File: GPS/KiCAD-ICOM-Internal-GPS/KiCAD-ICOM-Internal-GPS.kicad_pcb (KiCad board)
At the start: 2 copper layers, 20 x 35 mm, 2 parts, among them J1 ICOM-J1, U1 MAX-M10M-00B

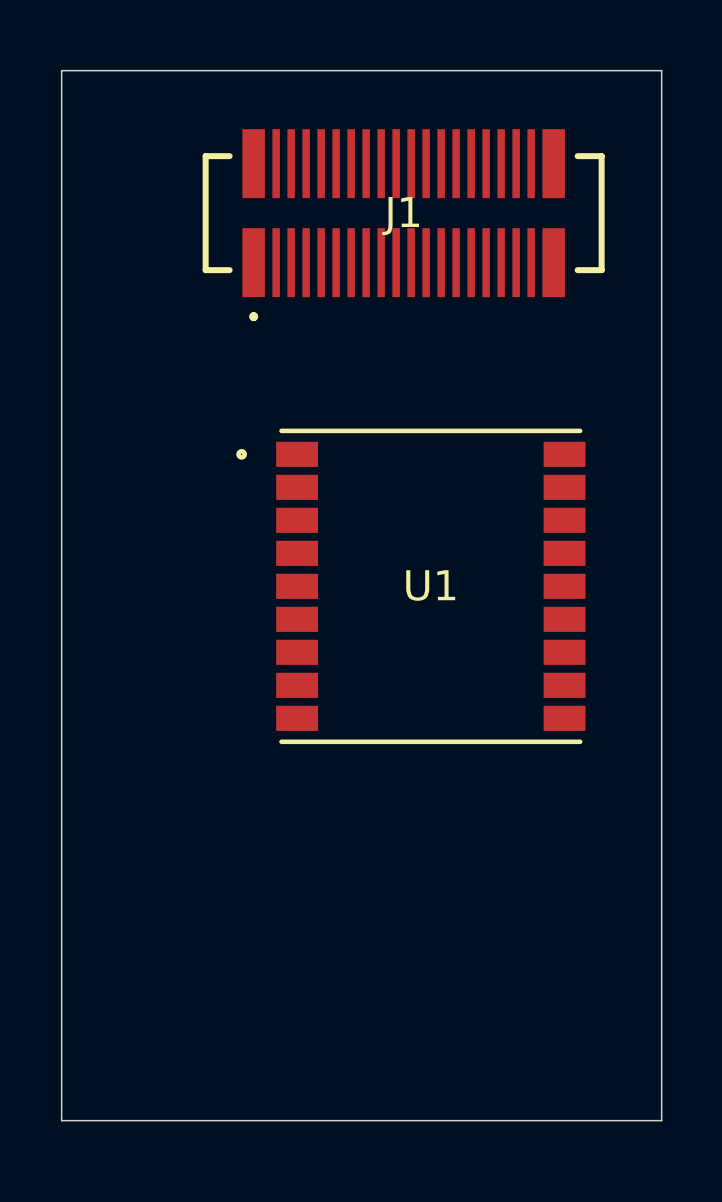
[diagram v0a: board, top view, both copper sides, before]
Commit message: updated v1.0 design
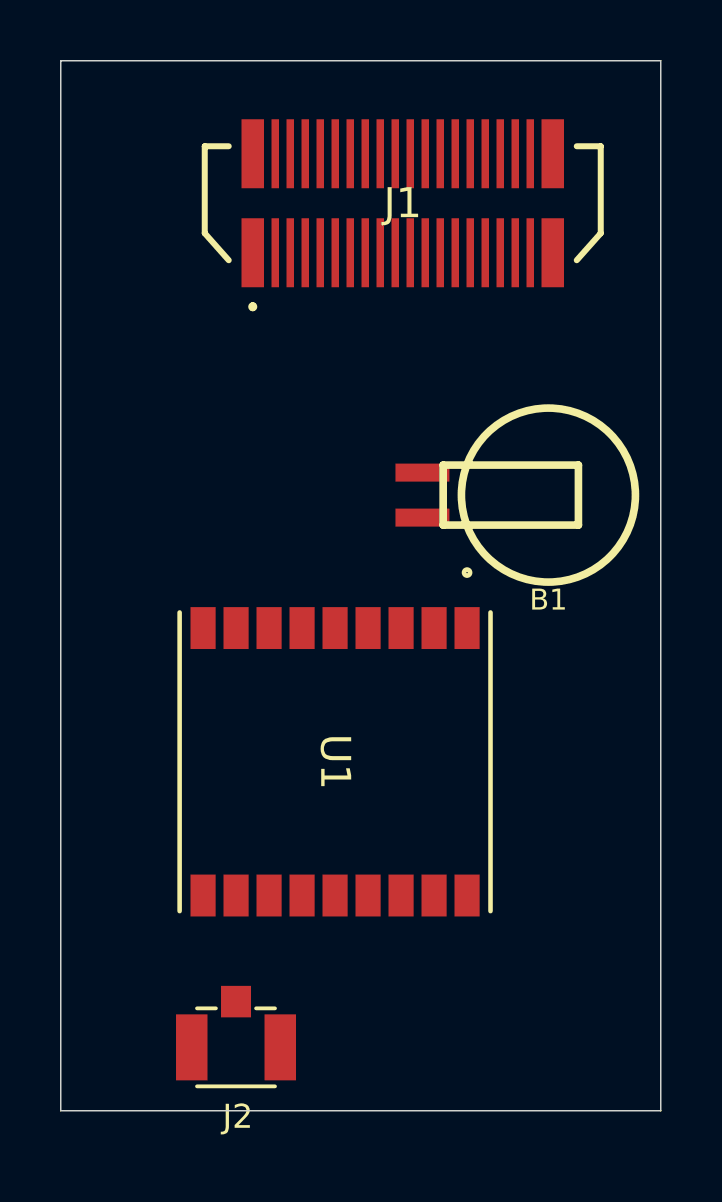
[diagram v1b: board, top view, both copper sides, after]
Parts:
- added B1: MS518SE, MS518SE:MS518SE-FL35E, F.Cu at (154.2, 93.2)
- added J2: U.FL-R-SMT-1_10_, U.FL-R-SMT-1_10:HRS_U.FL-R-SMT-1_10_, F.Cu at (143.8, 111.6)
- J1: footprint AXK640347YG:AXK640347YG -> ICOM-J1-J2:ICOM-J1-J2
- moved U1 6.66 mm to (147.1, 102.1), turned to -90 degrees
- moved J1 0.33 mm to (149.3, 83.5)
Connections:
- U1 pad 13: ANT-PWR-ON -> unconnected-(U1-LNA_EN-Pad13)
